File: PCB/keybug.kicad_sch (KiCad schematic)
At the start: 8 parts, among them U2 rp2040-zero

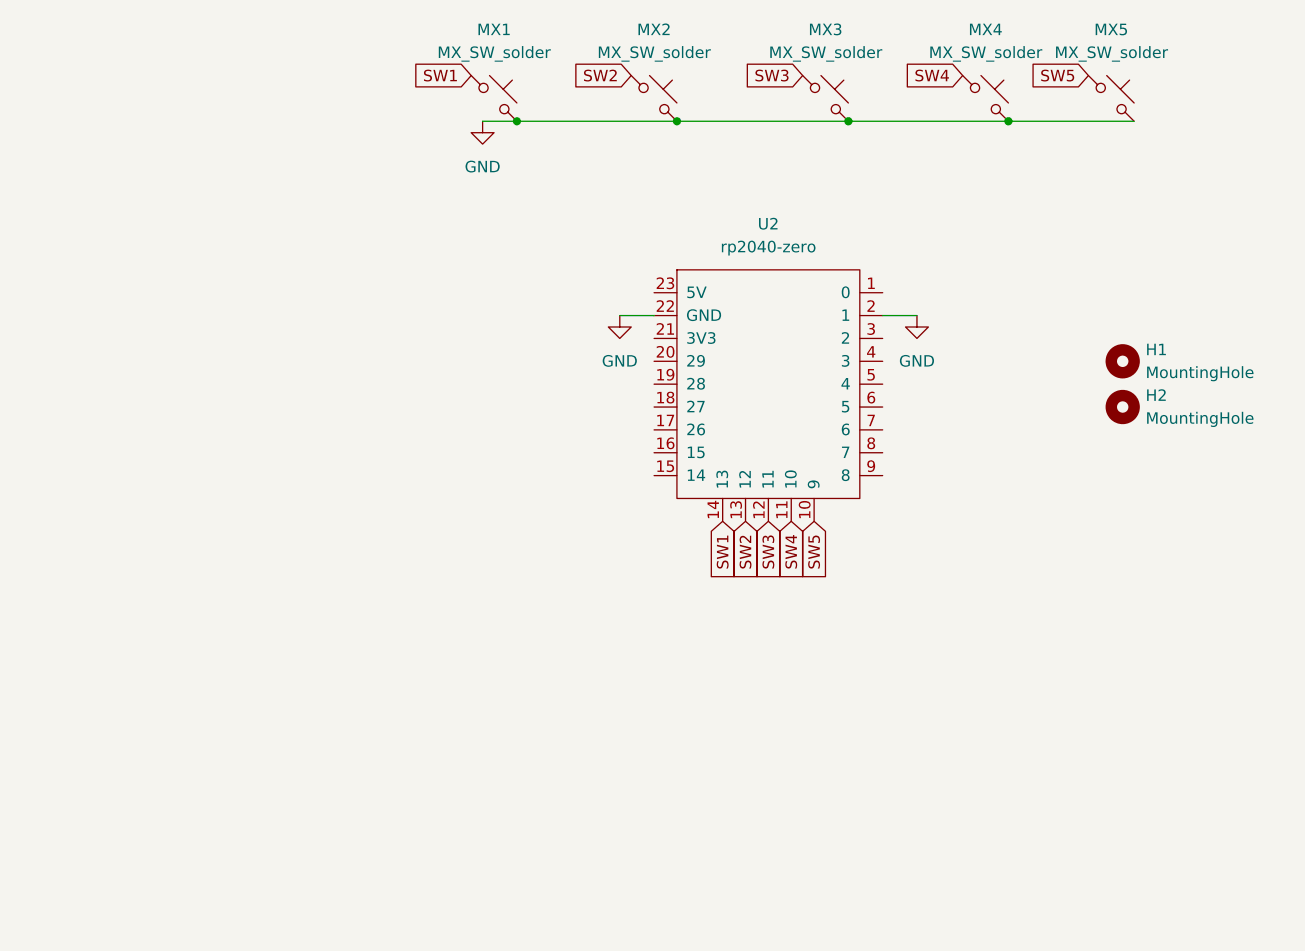
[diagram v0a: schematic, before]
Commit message: Add LEDs to PCB
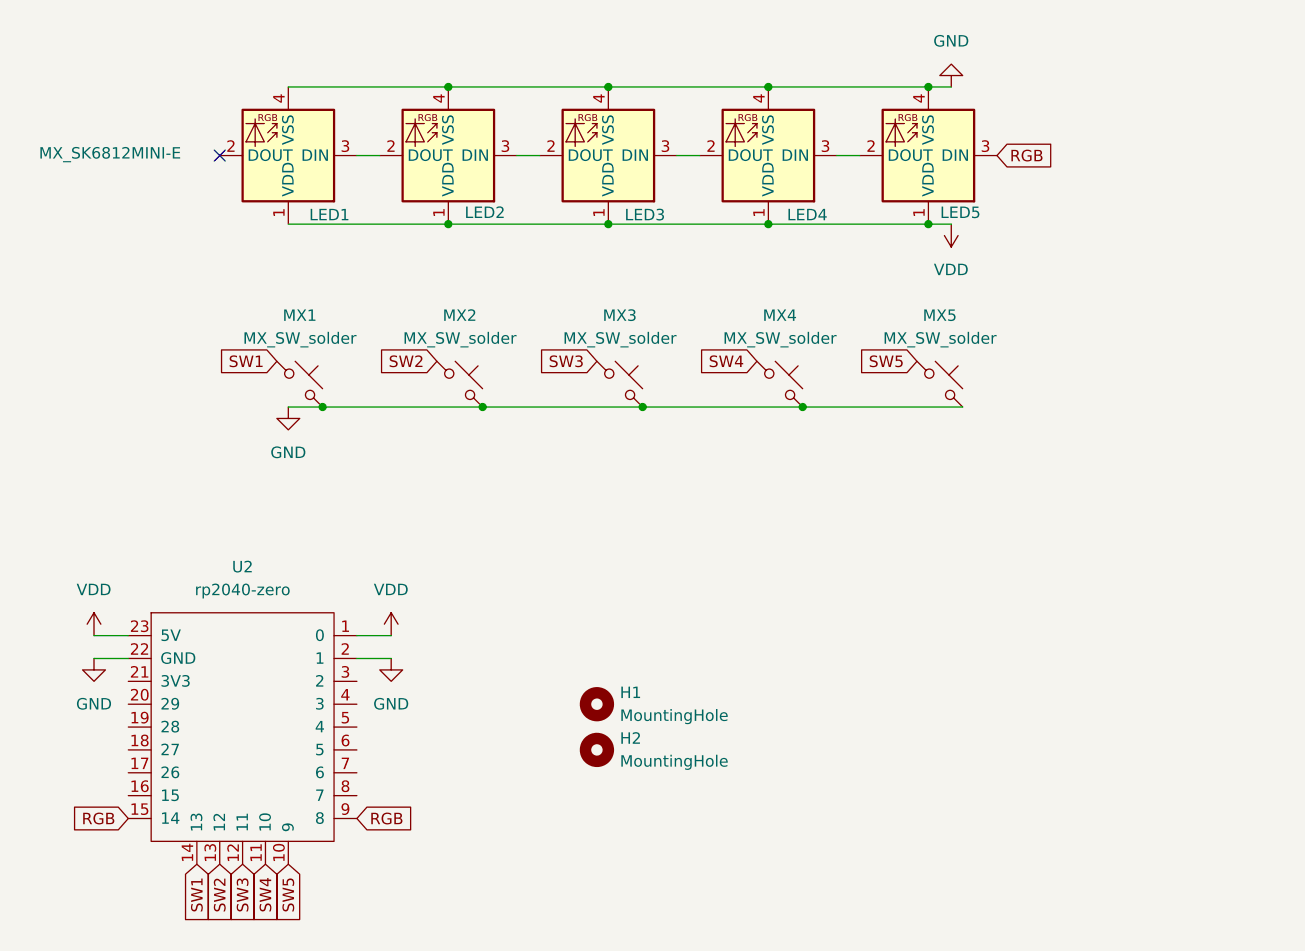
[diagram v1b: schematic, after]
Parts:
- added LED1, LED2, LED3, LED4, LED5: MX_SK6812MINI-E, PCM_marbastlib-mx:LED_MX_6028R-ROT, symbol PCM_marbastlib-mx:MX_SK6812MINI-E
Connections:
- net GND: now also LED1.4 (VSS), LED2.4 (VSS), LED3.4 (VSS), LED4.4 (VSS), LED5.4 (VSS)
- net VDD: now reaches U2.1 (0)
- net VDD: now also U2.23 (5V), LED1.1 (VDD), LED2.1 (VDD), LED3.1 (VDD), LED4.1 (VDD), LED5.1 (VDD)
- net RGB: now reaches U2.15 (14)
- net RGB: now also U2.9 (8), LED5.3 (DIN)
- new net: LED1.3 (DIN), LED2.2 (DOUT)
- new net: LED2.3 (DIN), LED3.2 (DOUT)
- new net: LED4.3 (DIN), LED5.2 (DOUT)
- new net: LED3.3 (DIN), LED4.2 (DOUT)
- no-connect marks 0 -> 1
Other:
- moved on the sheet: H1, H2, MX1, MX2, MX3, MX4, MX5, U2
